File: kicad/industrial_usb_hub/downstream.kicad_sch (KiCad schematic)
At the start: 4 parts, among them J1 USB_A, J3 USB_A, J4 USB_A, J5 USB_A

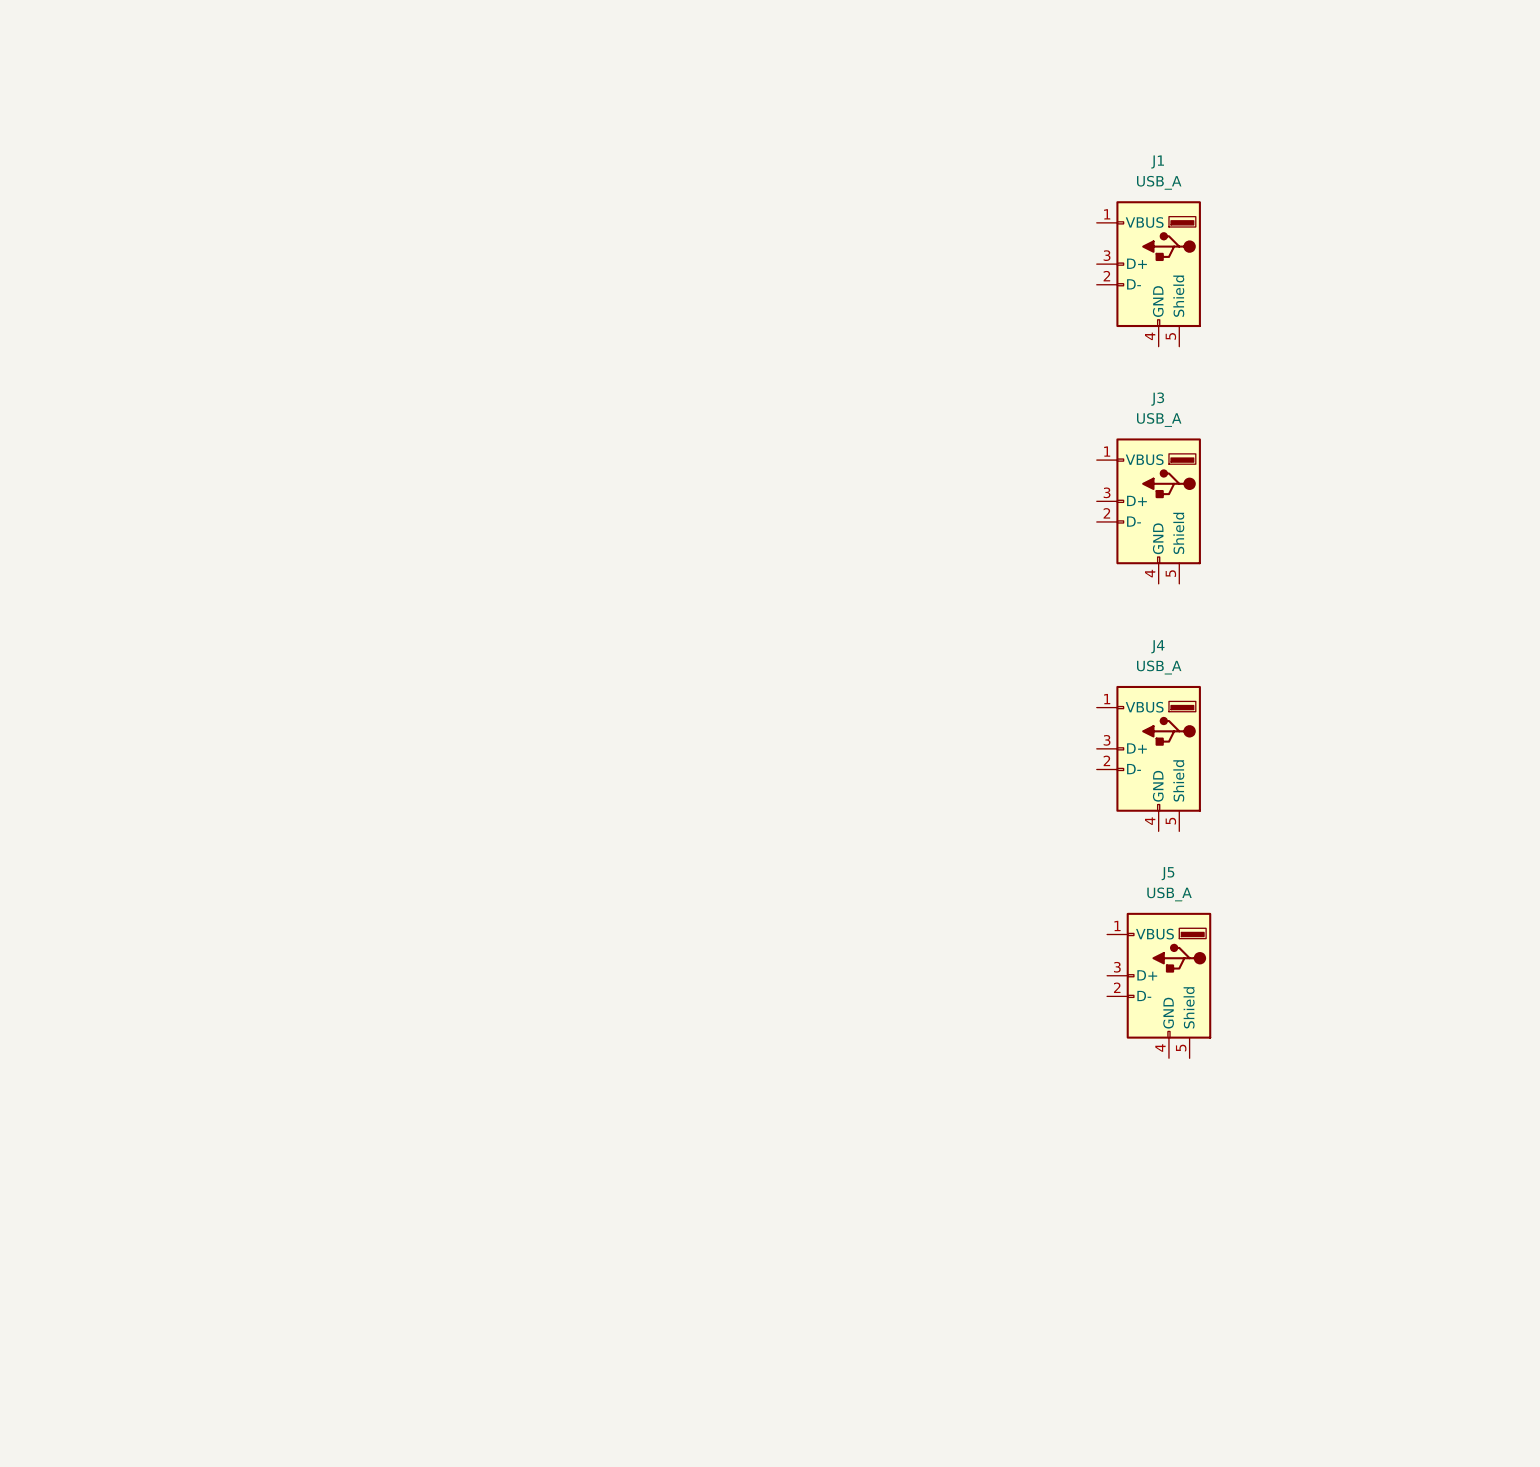
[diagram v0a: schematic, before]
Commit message: completed schematic
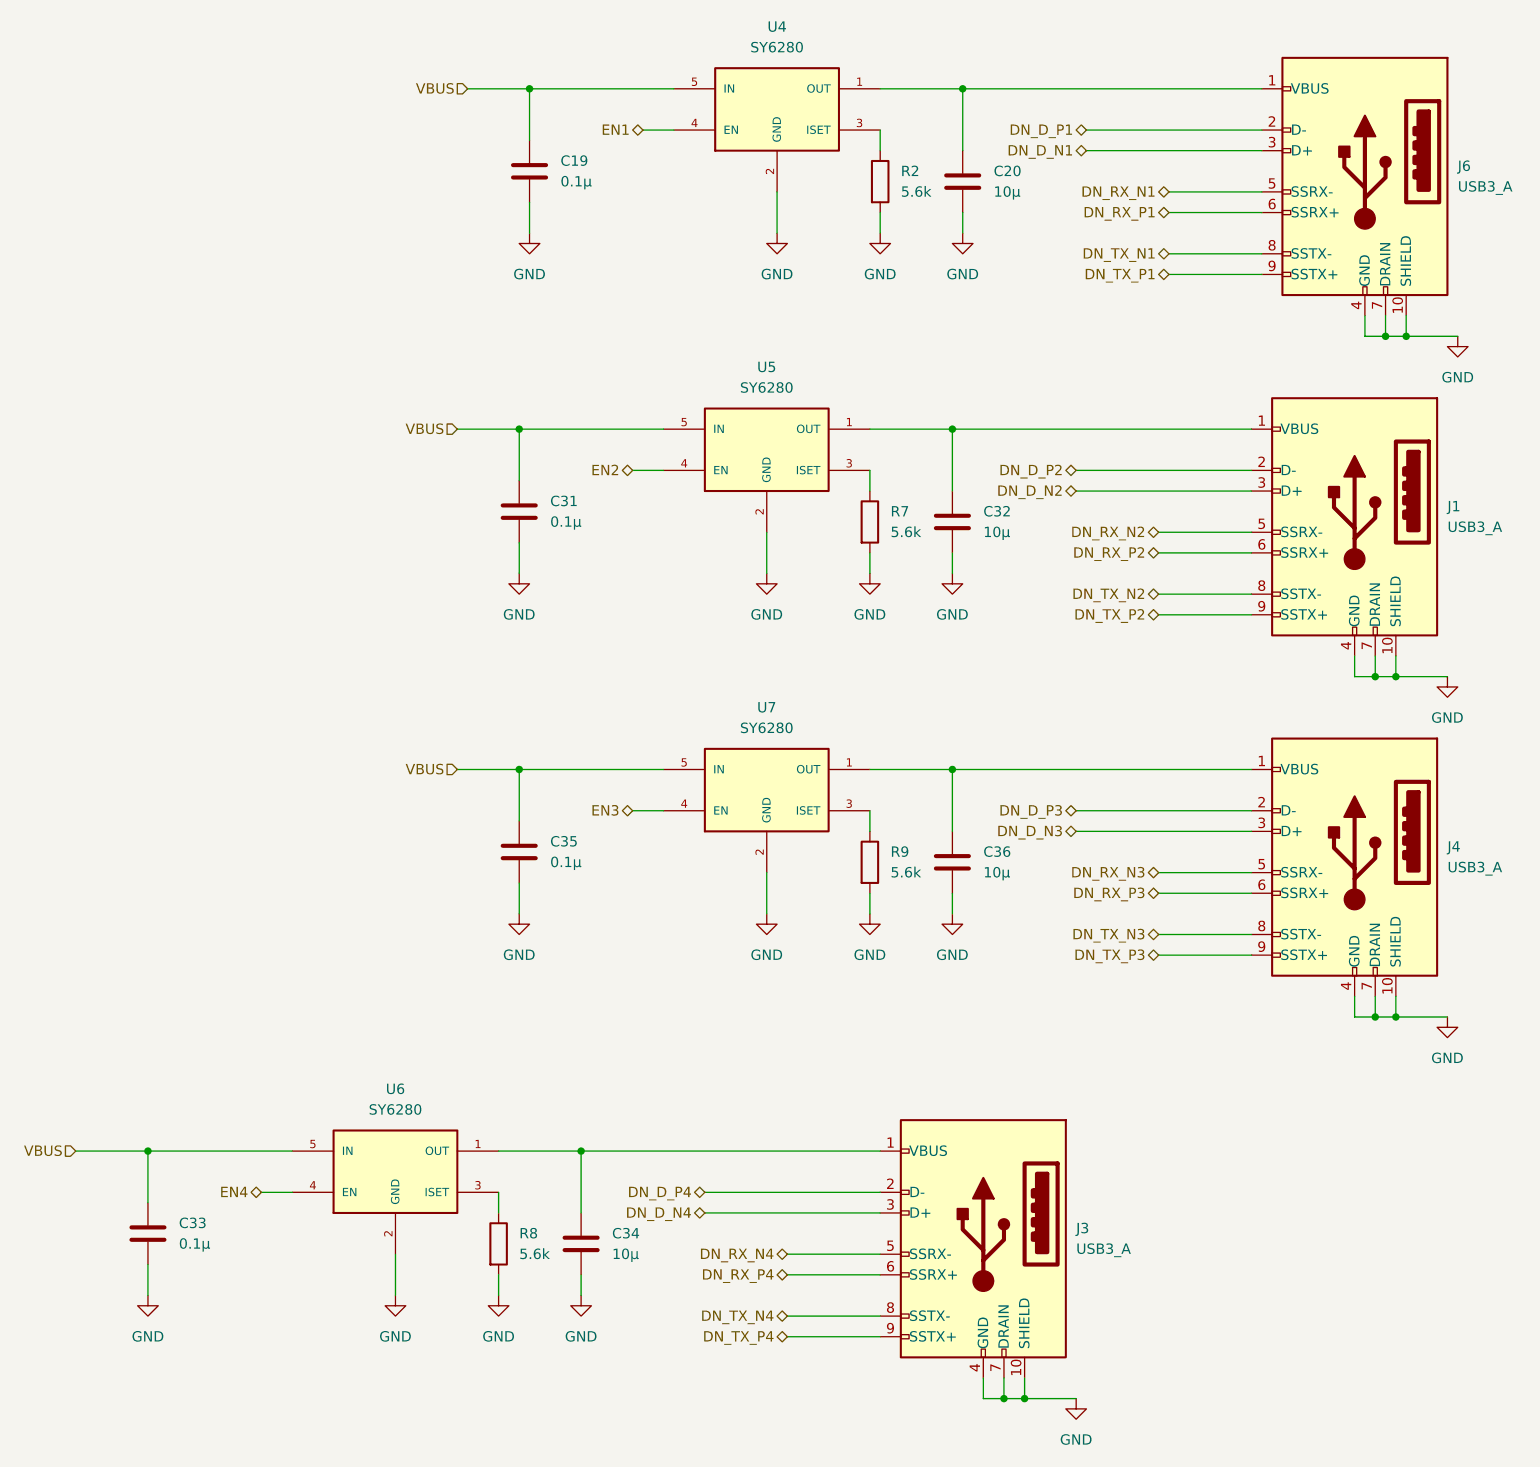
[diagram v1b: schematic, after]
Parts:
- removed J1, J3, J4, J5: USB_A, symbol Connector:USB_A
- added C19, C31, C33, C35: 0.1µ, Capacitor_SMD:C_0201_0603Metric, symbol Device:C
- added C20, C32, C34, C36: 10µ, Capacitor_SMD:C_0201_0603Metric, symbol Device:C
- added J1, J3, J4, J6: USB3_A, symbol Connector:USB3_A
- added R2, R7, R8, R9: 5.6k, symbol Device:R
- added U4, U5, U6, U7: SY6280, personal_library:SOT23-5, symbol SY6280:SY6280
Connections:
- new net: C34.2, J3.1 (VBUS), U6.1 (OUT)
- new net: R8.1, U6.3 (ISET)
- new net: C32.2, J1.1 (VBUS), U5.1 (OUT)
- new net: R7.1, U5.3 (ISET)
- new net: C20.2, J6.1 (VBUS), U4.1 (OUT)
- new net: R2.1, U4.3 (ISET)
- new net: C36.2, J4.1 (VBUS), U7.1 (OUT)
- new net: R9.1, U7.3 (ISET)
- new net DN_D_N1: J6.3 (D+)
- new net DN_D_N2: J1.3 (D+)
- new net DN_D_N3: J4.3 (D+)
- new net DN_D_N4: J3.3 (D+)
- new net DN_D_P1: J6.2 (D-)
- new net DN_D_P2: J1.2 (D-)
- new net DN_D_P3: J4.2 (D-)
- new net DN_D_P4: J3.2 (D-)
- new net DN_RX_N1: J6.5 (SSRX-)
- new net DN_RX_N2: J1.5 (SSRX-)
- new net DN_RX_N3: J4.5 (SSRX-)
- new net DN_RX_N4: J3.5 (SSRX-)
- new net DN_RX_P1: J6.6 (SSRX+)
- new net DN_RX_P2: J1.6 (SSRX+)
- new net DN_RX_P3: J4.6 (SSRX+)
- new net DN_RX_P4: J3.6 (SSRX+)
- new net DN_TX_N1: J6.8 (SSTX-)
- new net DN_TX_N2: J1.8 (SSTX-)
- new net DN_TX_N3: J4.8 (SSTX-)
- new net DN_TX_N4: J3.8 (SSTX-)
- new net DN_TX_P1: J6.9 (SSTX+)
- new net DN_TX_P2: J1.9 (SSTX+)
- new net DN_TX_P3: J4.9 (SSTX+)
- new net DN_TX_P4: J3.9 (SSTX+)
- new net EN1: U4.4 (EN)
- new net EN2: U5.4 (EN)
- new net EN3: U7.4 (EN)
- new net EN4: U6.4 (EN)
- new net GND: C19.1, C20.1, C31.1, C32.1, C33.1, C34.1, C35.1, C36.1, J1.10 (SHIELD), J1.4 (GND), J1.7 (DRAIN), J3.10 (SHIELD), J3.4 (GND), J3.7 (DRAIN), J4.10 (SHIELD), J4.4 (GND), J4.7 (DRAIN), J6.10 (SHIELD), J6.4 (GND), J6.7 (DRAIN), R2.2, R7.2, R8.2, R9.2, U4.2 (GND), U5.2 (GND), U6.2 (GND), U7.2 (GND)
- new net VBUS: C19.2, C31.2, C33.2, C35.2, U4.5 (IN), U5.5 (IN), U6.5 (IN), U7.5 (IN)
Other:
- title: (none) -> Downstream
